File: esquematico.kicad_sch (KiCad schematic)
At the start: 47 parts, among them J1 Screw_Terminal_01x02, J10 LCD I2C, J11 valvula, J2 BORNERA 1, J3 BORNERA 1, J4 BORNERA 2, J5 BORNERA 2, J6 BORNERA 1, J7 BORNERA 2, J8 BORNERA 1, J9 BORNERA 2, Q1 2N7000, Q2 2N7000, Q3 2N7000, Q4 2N7000, U1 PC817, U2 ESP32-DEVKITC-32D, U3 L7805, U4 PC817, U5 PC817, U6 PC817

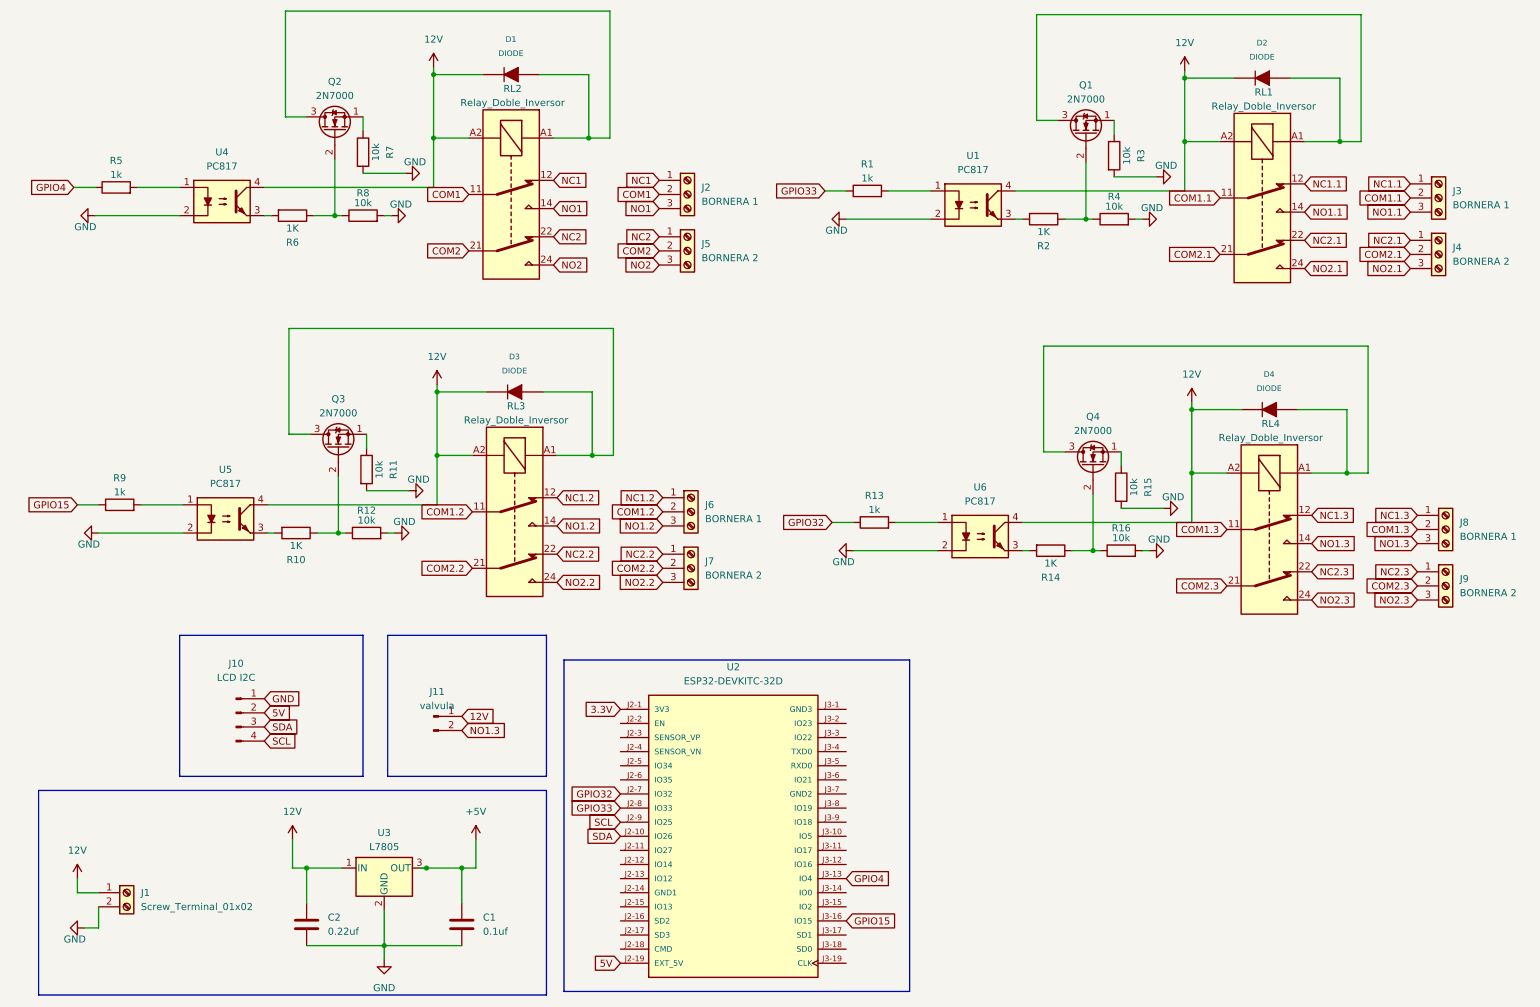
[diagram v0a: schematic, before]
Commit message: terminamos el pcb falta ordenar un poco mas
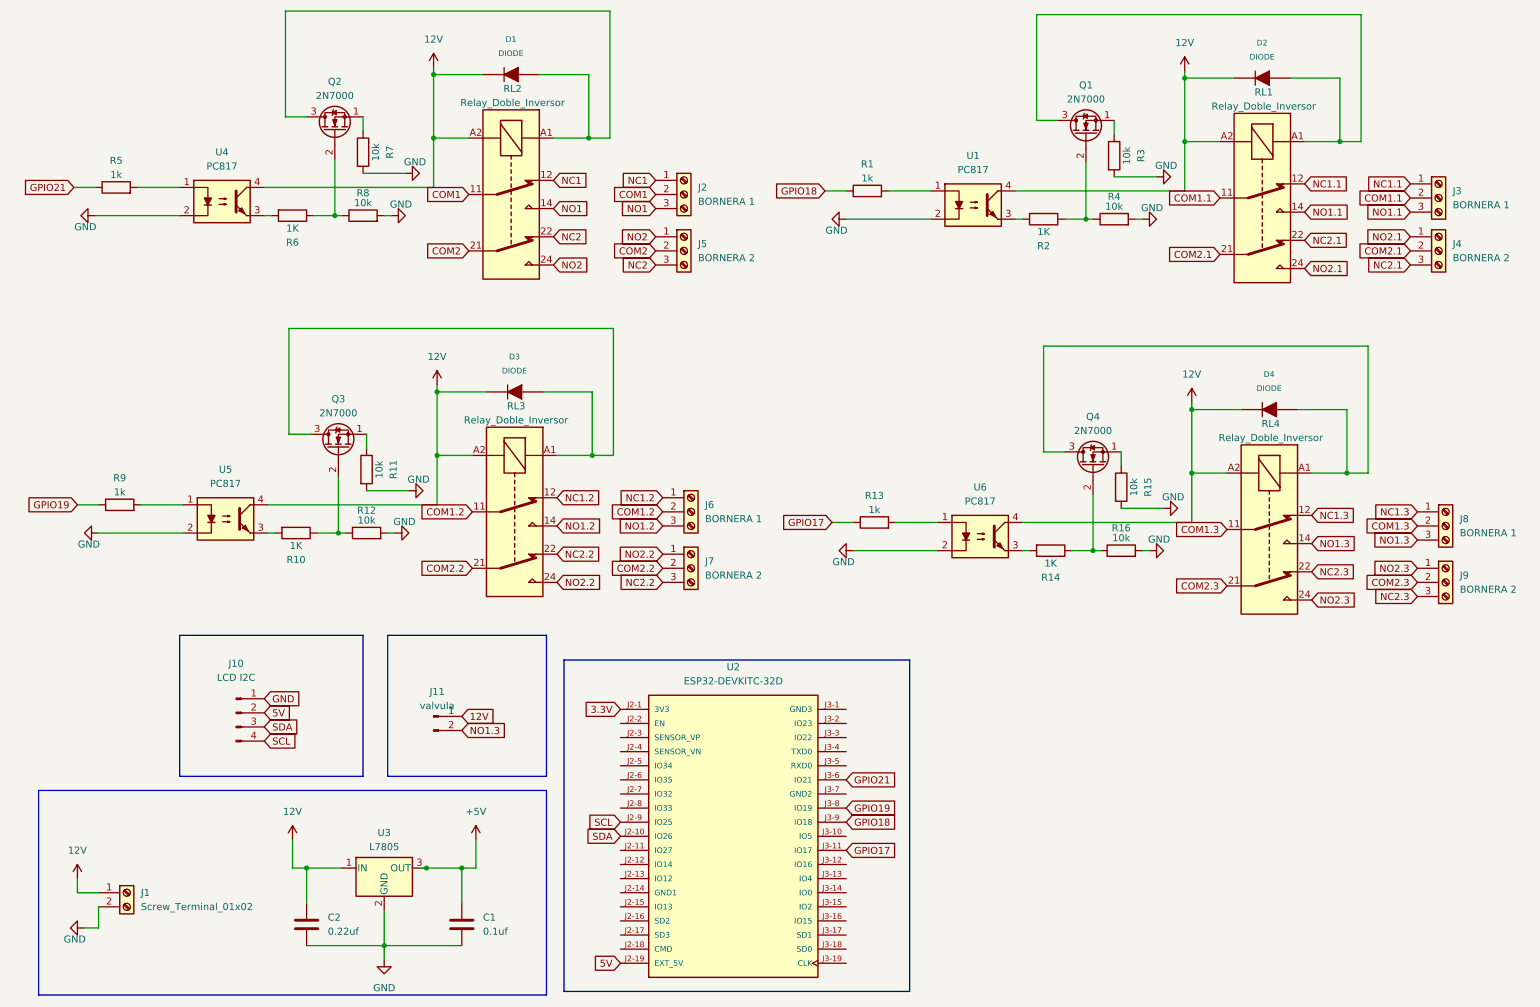
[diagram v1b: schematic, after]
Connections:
- net NC2: now also J5.3 (Pin_3); no longer J5.1 (Pin_1)
- net NC2.1: now also J4.3 (Pin_3); no longer J4.1 (Pin_1)
- net NC2.2: now also J7.3 (Pin_3); no longer J7.1 (Pin_1)
- net NC2.3: now also J9.3 (Pin_3); no longer J9.1 (Pin_1)
- net NO2: now also J5.1 (Pin_1); no longer J5.3 (Pin_3)
- net NO2.1: now also J4.1 (Pin_1); no longer J4.3 (Pin_3)
- net NO2.2: now also J7.1 (Pin_1); no longer J7.3 (Pin_3)
- net NO2.3: now also J9.1 (Pin_1); no longer J9.3 (Pin_3)
- net GPIO17: now reaches U2.J3-11 (IO17)
- net GPIO17: now also R13.1
- net GPIO21: now reaches U2.J3-6 (IO21)
- net GPIO21: now also R5.1
- net GPIO19: now reaches U2.J3-8 (IO19)
- net GPIO19: now also R9.1
- net GPIO18: now reaches U2.J3-9 (IO18)
- net GPIO18: now also R1.1
- net GPIO15: no longer names the net of U2.J3-16 (IO15)
- net GPIO15: no longer R9.1
- net GPIO32: no longer names the net of U2.J2-7 (IO32)
- net GPIO32: no longer R13.1
- net GPIO33: no longer names the net of U2.J2-8 (IO33)
- net GPIO33: no longer R1.1
- net GPIO4: no longer names the net of U2.J3-13 (IO4)
- net GPIO4: no longer R5.1
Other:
- moved on the sheet: J2, J4, J5, J8, J9
